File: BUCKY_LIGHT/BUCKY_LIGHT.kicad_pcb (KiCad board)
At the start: 4 copper layers, 145 x 130 mm, 134 parts, among them J1 LIGHT -> MAIN, Q1 Q_Photo_NPN, Q10 Q_Photo_NPN, Q11 Q_Photo_NPN, Q12 Q_Photo_NPN, Q13 Q_Photo_NPN, Q14 Q_Photo_NPN, Q15 Q_Photo_NPN, Q16 Q_Photo_NPN, Q17 Q_Photo_NPN, Q18 Q_Photo_NPN, Q19 Q_Photo_NPN, Q2 Q_Photo_NPN, Q20 Q_Photo_NPN, Q21 Q_Photo_NPN, Q22 Q_Photo_NPN, Q23 Q_Photo_NPN, Q24 Q_Photo_NPN, Q25 Q_Photo_NPN, Q26 Q_Photo_NPN, Q27 Q_Photo_NPN, Q28 Q_Photo_NPN, Q3 Q_Photo_NPN, Q4 Q_Photo_NPN, Q5 Q_Photo_NPN, Q6 Q_Photo_NPN, Q7 Q_Photo_NPN, Q8 Q_Photo_NPN, Q9 Q_Photo_NPN

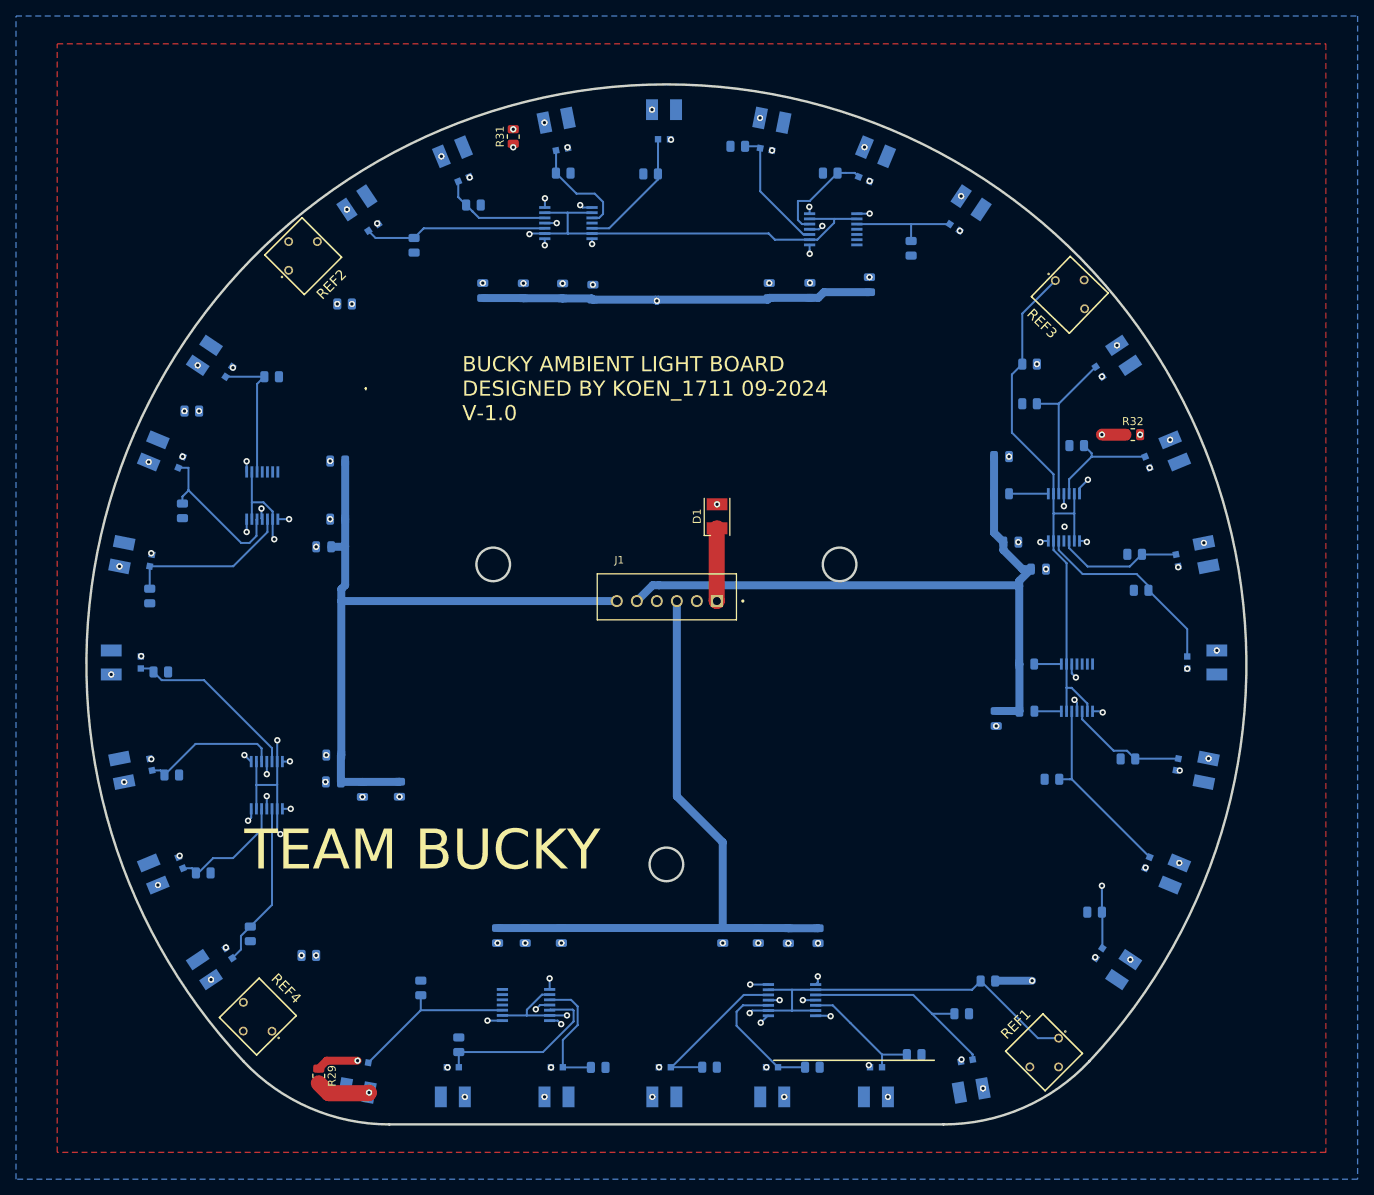
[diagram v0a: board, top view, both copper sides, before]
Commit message: fix: BUCKY_MAIN v2?
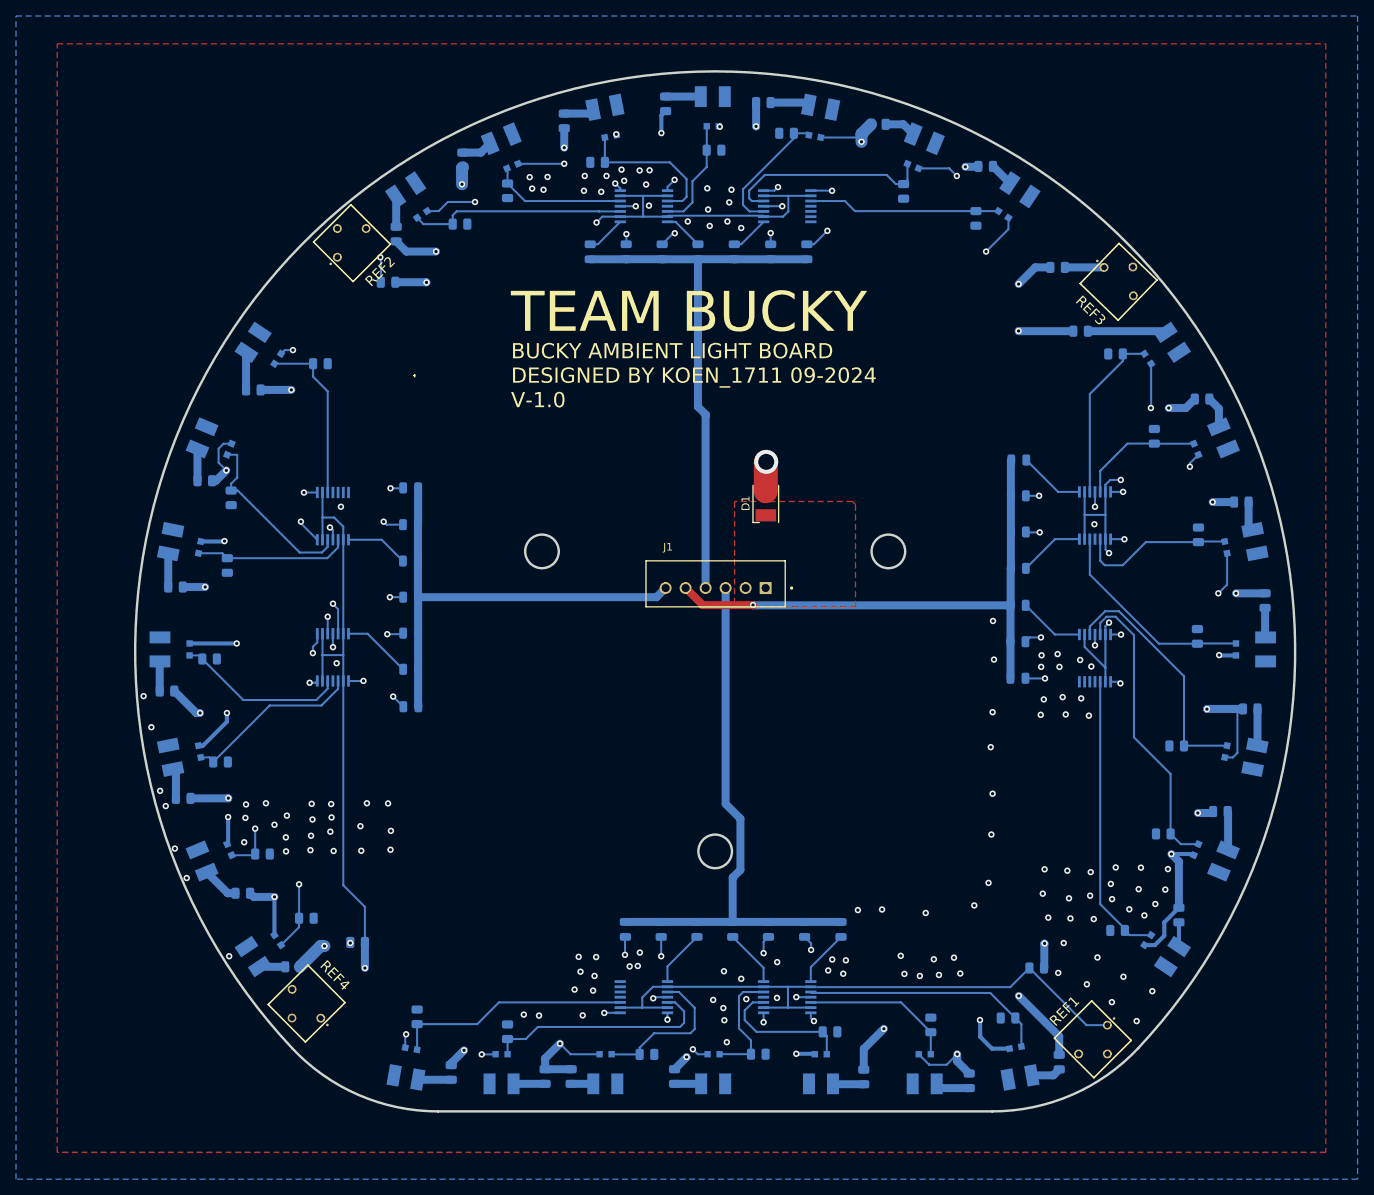
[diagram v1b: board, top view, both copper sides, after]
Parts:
- added R34: 10k, Resistor_SMD:R_0805_2012Metric, B.Cu at (128.1, 156.7)
- added R36: 10k, Resistor_SMD:R_0805_2012Metric, B.Cu at (96.6, 143.0)
- added R38: 10k, Resistor_SMD:R_0805_2012Metric, B.Cu at (82.9, 121.9)
- added R40: 10k, Resistor_SMD:R_0805_2012Metric, B.Cu at (81.9, 95.5)
- added R41: 10k, Resistor_SMD:R_0805_2012Metric, B.Cu at (85.6, 82.2)
- added R42: 10k, Resistor_SMD:R_0805_2012Metric, B.Cu at (91.7, 70.9)
- added R43: 10k, Resistor_SMD:R_0805_2012Metric, B.Cu at (109.5, 51.4)
- added R44: 10k, Resistor_SMD:R_0805_2012Metric, B.Cu at (117.9, 42.1)
- added R45: 10k, Resistor_SMD:R_0805_2012Metric, B.Cu at (130.5, 37.3)
- added R46: 10k, Resistor_SMD:R_0805_2012Metric, B.Cu at (143.2, 35.1)
- added R47: 10k, Resistor_SMD:R_0805_2012Metric, B.Cu at (155.4, 35.0)
- added R48: 10k, Resistor_SMD:R_0805_2012Metric, B.Cu at (169.8, 37.7)
- added R49: 10k, Resistor_SMD:R_0805_2012Metric, B.Cu at (183.2, 43.0)
- added R50: 10k, Resistor_SMD:R_0805_2012Metric, B.Cu at (195.1, 63.6)
- added R51: 10k, Resistor_SMD:R_0805_2012Metric, B.Cu at (210.3, 72.0)
- added R52: 10k, Resistor_SMD:R_0805_2012Metric, B.Cu at (215.2, 84.9)
- added R53: 10k, Resistor_SMD:R_0805_2012Metric, B.Cu at (218.1, 97.2)
- added R54: 10k, Resistor_SMD:R_0805_2012Metric, B.Cu at (216.3, 110.8)
- added R55: 10k, Resistor_SMD:R_0805_2012Metric, B.Cu at (212.5, 123.6)
- added R56: 10k, Resistor_SMD:R_0805_2012Metric, B.Cu at (207.4, 136.5)
- added R57: 20k, Resistor_SMD:R_0805_2012Metric, B.Cu at (189.6, 143.2)
- added R58: 20k, Resistor_SMD:R_0805_2012Metric, B.Cu at (108.5, 57.4)
- added R59: 20k, Resistor_SMD:R_0805_2012Metric, B.Cu at (192.2, 55.6)
- added R60: 20k, Resistor_SMD:R_0805_2012Metric, B.Cu at (104.7, 140.0)
- R29, R31, R32: moved to B.Cu
- R33, R35, R37, R39: value 20k -> 10k
- moved R30 128.3 mm to (181.2, 157.2), turned to -90 degrees
- moved R31 125.5 mm to (168.0, 156.8), turned to -90 degrees
- moved R37 118.5 mm to (90.3, 133.8)
- moved R32 98.6 mm to (144.3, 156.7), turned to -90 degrees
- moved R35 97.0 mm to (116.4, 156.2), turned to -90 degrees
- moved R29 92.6 mm to (192.4, 154.9)
- moved R33 53.4 mm to (131.4, 156.7), turned to -90 degrees
- moved R39 37.5 mm to (80.9, 108.5), turned to 180 degrees
- moved LI11 25.0 mm to (111.3, 96.8)
- moved LI5 21.5 mm to (147.1, 138.3)
- moved LI16 18.6 mm to (138.3, 53.6)
- moved LI17 18.0 mm to (142.8, 53.6)
- moved LI10 18.0 mm to (111.3, 101.3)
- moved COMP3 18.0 mm to (101.6, 104.3), turned to -90 degrees
- moved LI7 16.0 mm to (138.2, 138.3)
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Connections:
- L11 pad 2: Net-(L10-A) -> Net-(L11-A)
- L12 pad 2: Net-(L10-A) -> Net-(L12-A)
- L13 pad 2: Net-(L10-A) -> Net-(L13-A)
- L14 pad 2: Net-(L10-A) -> Net-(L14-A)
- L16 pad 2: Net-(L15-A) -> Net-(L16-A)
- L17 pad 2: Net-(L15-A) -> Net-(L17-A)
- L18 pad 2: Net-(L15-A) -> Net-(L18-A)
- L19 pad 2: Net-(L15-A) -> Net-(L19-A)
- L2 pad 2: Net-(L1-A) -> Net-(L2-A)
- L20 pad 2: Net-(L15-A) -> Net-(L20-A)
- L21 pad 2: Net-(L15-A) -> Net-(L21-A)
- L23 pad 2: Net-(L22-A) -> Net-(L23-A)
- L24 pad 2: Net-(L22-A) -> Net-(L24-A)
- L25 pad 2: Net-(L22-A) -> Net-(L25-A)
- L26 pad 2: Net-(L22-A) -> Net-(L26-A)
- L27 pad 2: Net-(L22-A) -> Net-(L27-A)
- L28 pad 2: Net-(L22-A) -> Net-(L28-A)
- L3 pad 2: Net-(L1-A) -> Net-(L3-A)
- L4 pad 2: Net-(L1-A) -> Net-(L4-A)
- L5 pad 2: Net-(L1-A) -> Net-(L5-A)
- L6 pad 2: Net-(L1-A) -> Net-(L6-A)
- L7 pad 2: Net-(L1-A) -> Net-(L7-A)
- L8 pad 2: Net-(L10-A) -> Net-(L8-A)
- L9 pad 2: Net-(L10-A) -> Net-(L9-A)
- R30 pad 2: Net-(L10-A) -> Net-(L2-A)
- R31 pad 2: Net-(L15-A) -> Net-(L3-A)
- R32 pad 2: Net-(L22-A) -> Net-(L4-A)
- R33 pad 2: /TRES_FRONT_I -> Net-(L5-A)
- R35 pad 2: /TRES_BACK_I -> Net-(L7-A)
- R37 pad 2: /TRES_LEFT_I -> Net-(L9-A)
- R39 pad 2: /TRES_RIGHT_I -> Net-(L11-A)
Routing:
- net +5V: track 587.7 -> 1181.6 mm, vias 44 -> 60
- net Net-(L10-A): track 89.7 -> 3.82 mm, vias 8 -> 0
- net Net-(L15-A): track 86.4 -> 3.72 mm, vias 8 -> 0
- net Net-(L22-A): track 90.5 -> 9.79 mm, vias 8 -> 0
- net Net-(L1-A): track 84.2 -> 3.74 mm, vias 7 -> 0
- net /ANALOG_COMP_RIGHT/I2: track 15.0 -> 42.9 mm, vias 0 -> 2
- net /ANALOG_COMP_RIGHT/I1: track 20.7 -> 46.5 mm, vias 0 -> 2
- net /SIG_RIGHT: track 83.9 -> 58.8 mm
- net /SIG_BACK: track 86.5 -> 68.6 mm, vias 1 -> 0
- net /SIG_LEFT: track 86.5 -> 68.9 mm, vias 0 -> 1
- net /ANALOG_COMP_LEFT/I5: track 15.1 -> 31.0 mm
- net Net-(COMP3-OUT_D): track 6.46 -> 21.4 mm
- net /ANALOG_COMP_LEFT/I6: track 23.8 -> 37.7 mm
- net /SIG_FRONT: track 83.3 -> 69.9 mm
- net Net-(COMP3-OUT_B): track 21.8 -> 8.67 mm, vias 2 -> 0
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- added copper zone on F.Cu, net Net-(D1-A)
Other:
- board text removed: "BUCKY AMBIENT LIGHT BOARD DESIGNED BY KOEN_1711 08-2024 V-1.0"
